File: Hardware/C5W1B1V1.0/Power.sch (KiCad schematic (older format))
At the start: 10 parts, among them IC2 USBLC6-2P6, J5 USB4105GFA120, U9 LD1117S33TR_SOT223

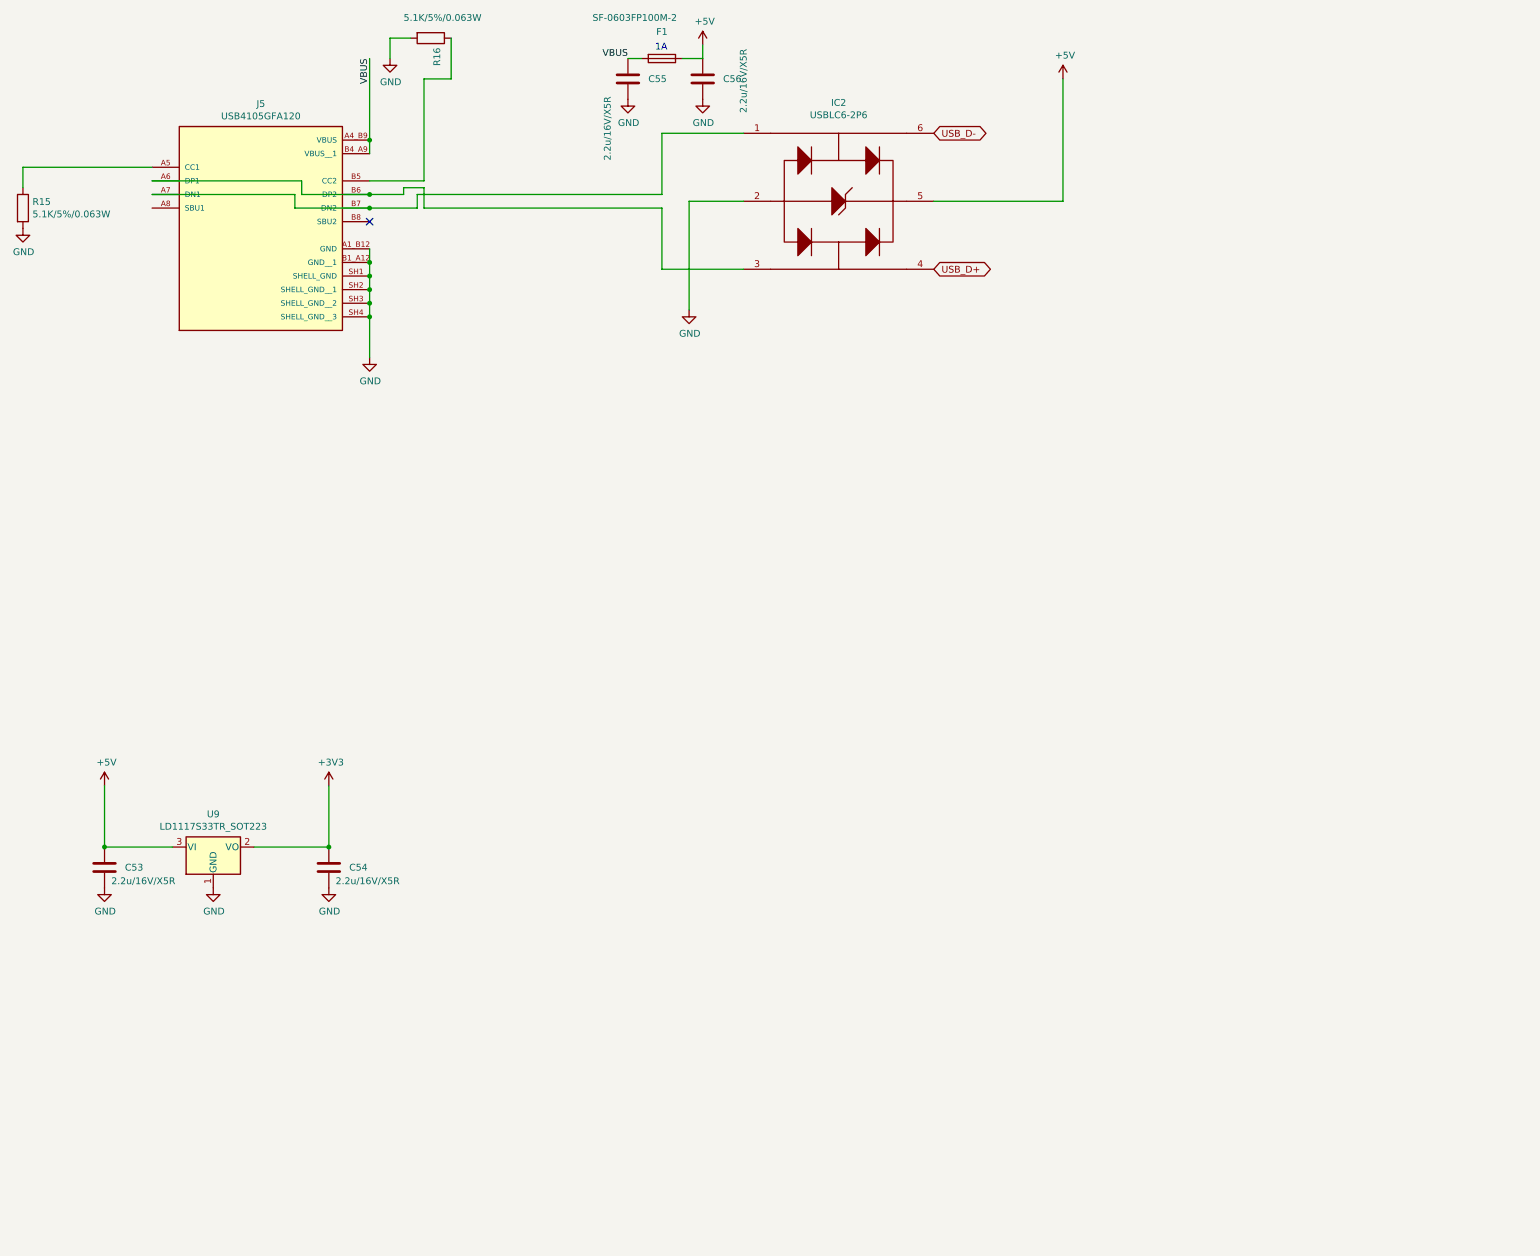
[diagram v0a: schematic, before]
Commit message: Rozlana masa
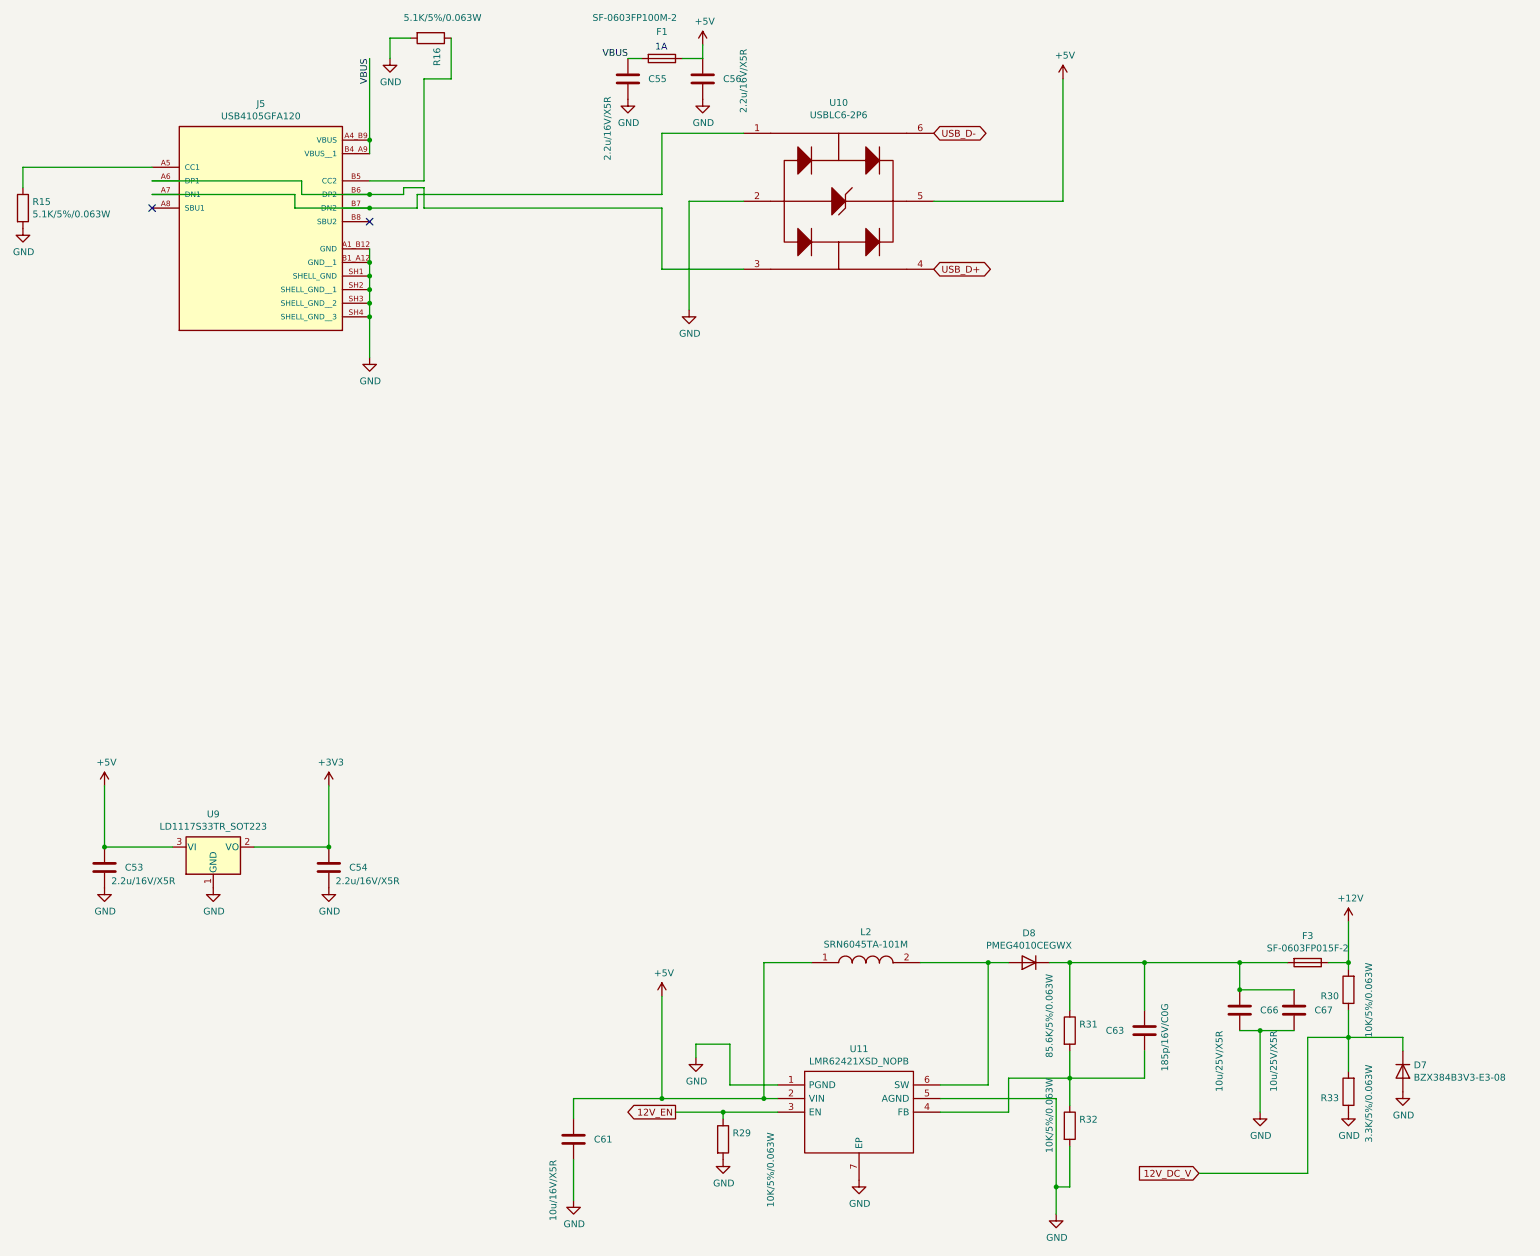
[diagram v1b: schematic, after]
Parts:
- added C61: 10u/16V/X5R, Capacitor_SMD:C_0603_1608Metric, symbol Device:C
- added C63: 185p/16V/C0G, Capacitor_SMD:C_0402_1005Metric, symbol Device:C
- added C66, C67: 10u/25V/X5R, Capacitor_SMD:C_1206_3216Metric, symbol Device:C
- added D7: BZX384B3V3-E3-08, Diode_SMD:D_SOD-323, symbol Device:D
- added D8: PMEG4010CEGWX, Diode_SMD:D_SOD-123, symbol Device:D
- added F3: SF-0603FP015F-2, Fuse:Fuse_0603_1608Metric, symbol Device:Fuse
- added L2: SRN6045TA-101M, SRN6045TA220M, symbol SRN6045TA-101M:SRN6045TA-101M
- added R29, R30, R32: 10K/5%/0.063W, Resistor_SMD:R_0402_1005Metric, symbol Device:R
- added R31: 85.6K/5%/0.063W, Resistor_SMD:R_0402_1005Metric, symbol Device:R
- added R33: 3.3K/5%/0.063W, Resistor_SMD:R_0402_1005Metric, symbol Device:R
- added U11: LMR62421XSD_NOPB, SON95P300X300X80-7N, symbol LMR62421XSD_NOPB:LMR62421XSD_NOPB
- renumbered IC2 to U10
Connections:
- net +5V: now also C61.1, L2.1, U11.2 (VIN)
- net GND: now also C61.2, C66.2, C67.2, D7.2 (A), R29.2, R32.2, R33.1, U11.1 (PGND), U11.5 (AGND), U11.7 (EP)
- new net: C63.1, R31.2, R32.1, U11.4 (FB)
- new net: D8.2 (A), L2.2, U11.6 (SW)
- new net: C63.2, C66.1, C67.1, D8.1 (K), F3.2, R31.1
- new net +12V: F3.1, R30.2
- new net 12V_DC_V: D7.1 (K), R30.1, R33.2
- new net 12V_EN: R29.1, U11.3 (EN)
- no-connect marks 1 -> 2

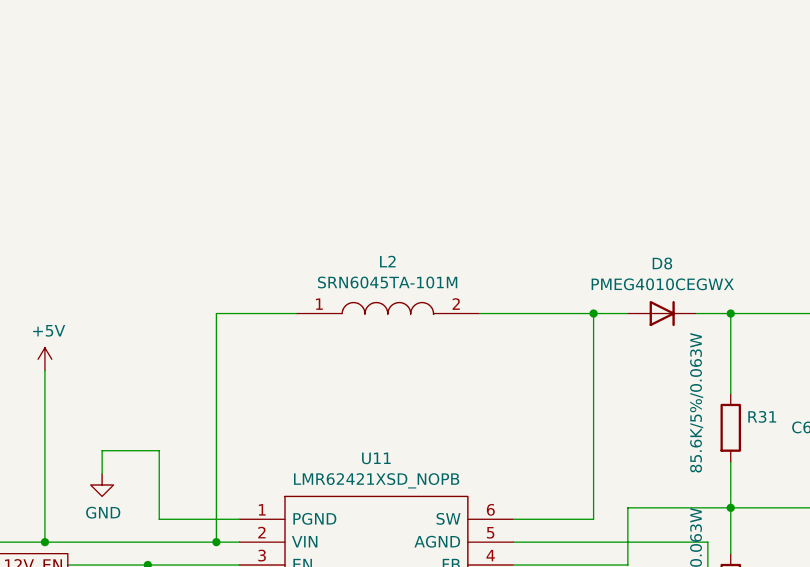
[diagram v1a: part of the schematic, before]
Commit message: End PCB
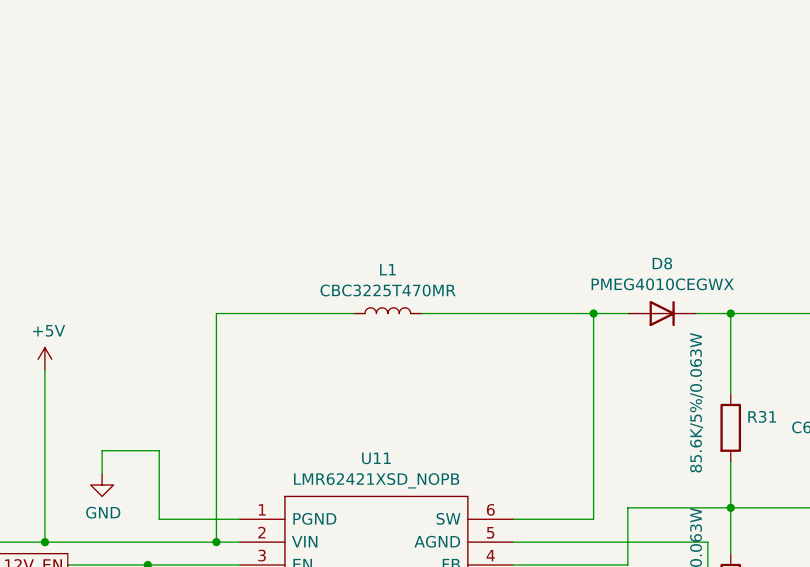
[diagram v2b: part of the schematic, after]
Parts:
- removed L2: SRN6045TA-101M, SRN6045TA220M, symbol SRN6045TA-101M:SRN6045TA-101M
- added L1: CBC3225T470MR, Inductor_SMD:L_1210_3225Metric, symbol Device:L
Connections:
- net +5V: now also L1.1
- net at D8.2 (A), U11.6 (SW): now also L1.2
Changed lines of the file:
@@
 Connection ~ 9050 7750
-Wire Wire Line
-	8550 7750 9050 7750
-Wire Wire Line
-	7400 7750 7750 7750
 Wire Wire Line
 	7400 8750 7400 7750
@@
 Wire Wire Line
 	6000 8750 6000 8900
-$Comp
-L SRN6045TA-101M:SRN6045TA-101M L2
-U 1 1 6683B75C
-P 7750 7750
-F 0 "L2" H 8150 7975 50  0000 C CNN
-F 1 "SRN6045TA-101M" H 8150 7884 50  0000 C CNN
-F 2 "SRN6045TA220M" H 8400 7800 50  0001 L CNN
-F 3 "https://www.bourns.com/docs/Product-Datasheets/SRN6045TA.pdf" H 8400 7700 50  0001 L CNN
-F 4 "fixed Inductor 100uH 0.82A Shielded" H 8400 7600 50  0001 L CNN "Description"
-F 5 "4" H 8400 7500 50  0001 L CNN "Height"
-F 6 "Bourns" H 8400 7400 50  0001 L CNN "Manufacturer_Name"
-F 7 "SRN6045TA-101M" H 8400 7300 50  0001 L CNN "Manufacturer_Part_Number"
-F 8 "652-SRN6045TA-101M" H 8400 7200 50  0001 L CNN "Mouser Part Number"
-F 9 "https://www.mouser.co.uk/ProductDetail/Bourns/SRN6045TA-101M?qs=Vt59ZOdFuWaW81VrtId3eg%3D%3D" H 8400 7100 50  0001 L CNN "Mouser Price/Stock"
-F 10 "SRN6045TA-101M" H 8400 7000 50  0001 L CNN "Arrow Part Number"
-F 11 "https://www.arrow.com/en/products/srn6045ta-101m/bourns?region=nac" H 8400 6900 50  0001 L CNN "Arrow Price/Stock"
-	1    7750 7750
-	1    0    0    -1
-$EndComp
 $Comp
 L power:GND #PWR0249
@@
 Wire Wire Line
 	10600 9300 11400 9300
+$Comp
+L Device:L L1
+U 1 1 66BF236E
+P 8150 7750
+F 0 "L1" V 8340 7750 50  0000 C CNN
+F 1 "CBC3225T470MR" V 8249 7750 50  0000 C CNN
+F 2 "Inductor_SMD:L_1210_3225Metric" H 8150 7750 50  0001 C CNN
+F 3 "~" H 8150 7750 50  0001 C CNN
+	1    8150 7750
+	0    -1   -1   0
+$EndComp
+Wire Wire Line
+	7400 7750 8000 7750
+Wire Wire Line
+	8300 7750 9050 7750
 $EndSCHEMATC
